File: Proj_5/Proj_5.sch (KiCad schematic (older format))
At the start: 0 parts

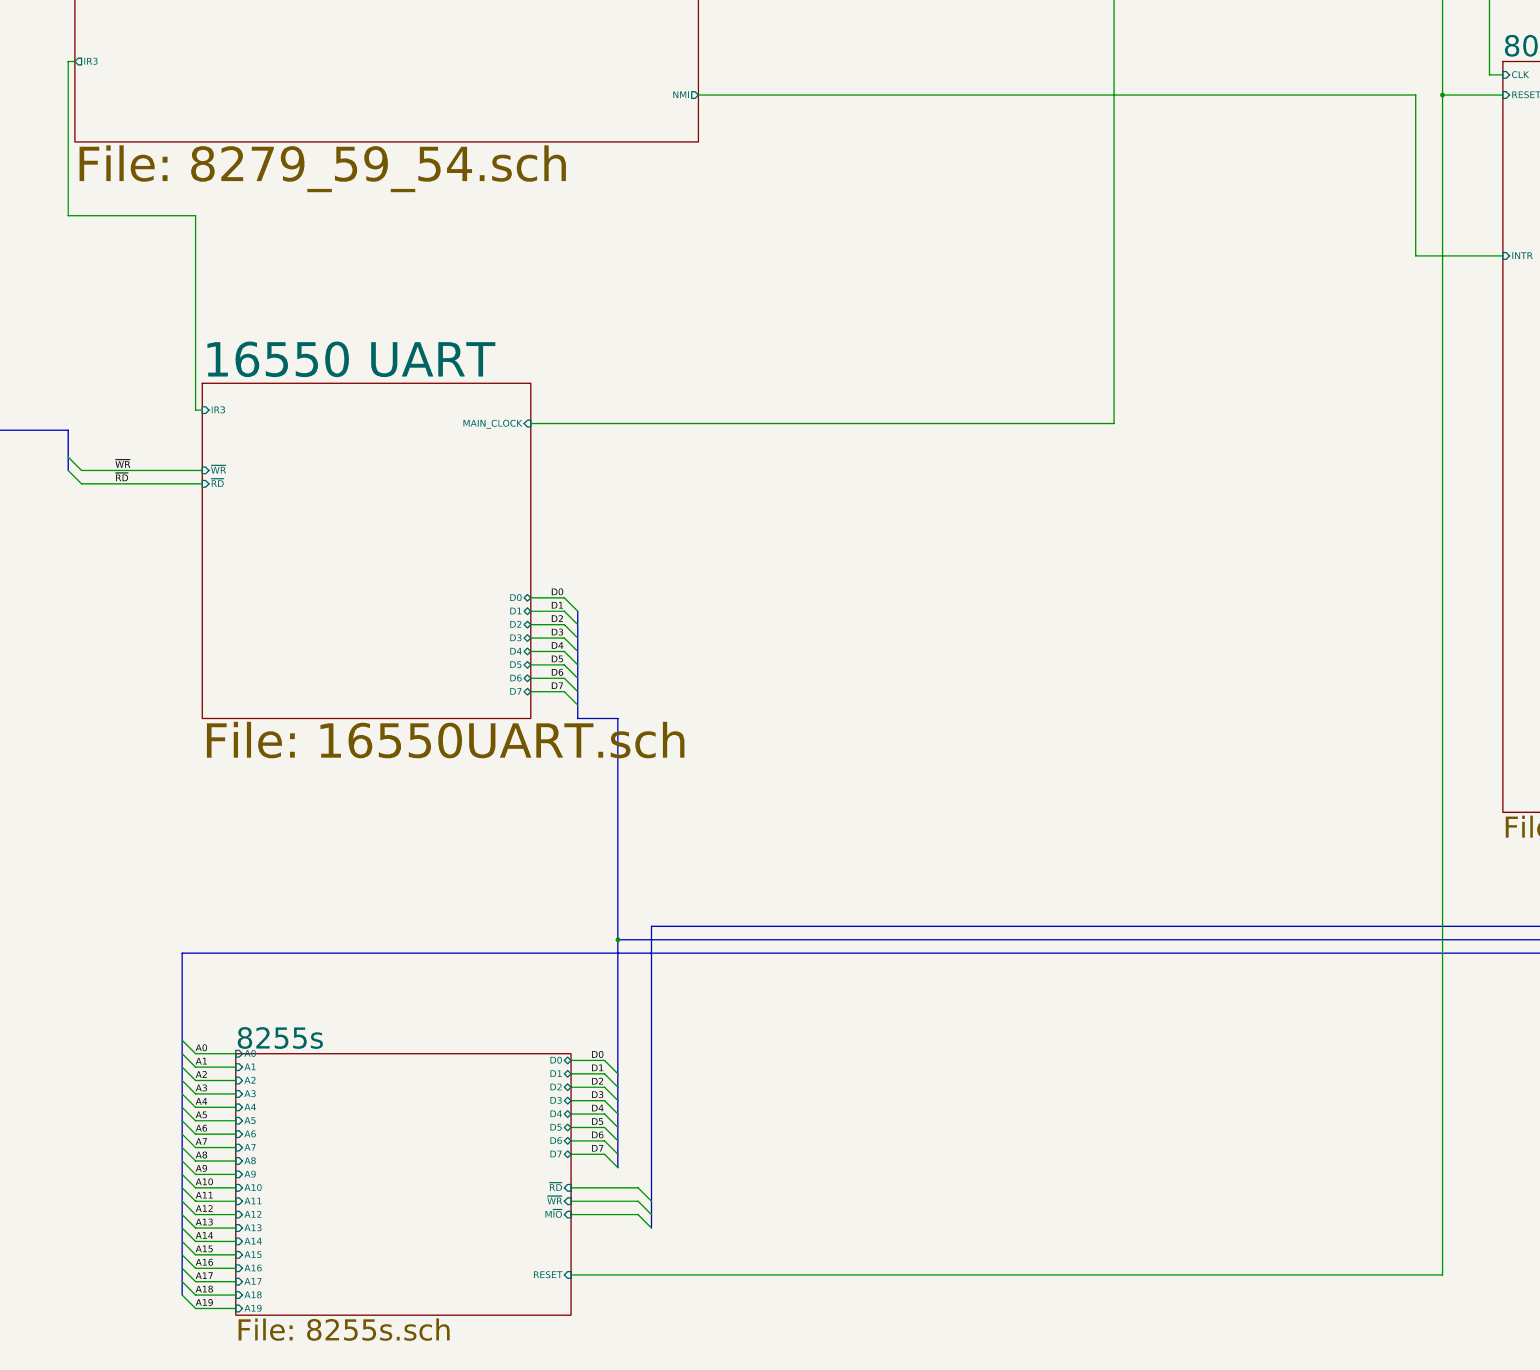
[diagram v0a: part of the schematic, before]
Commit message: Monch
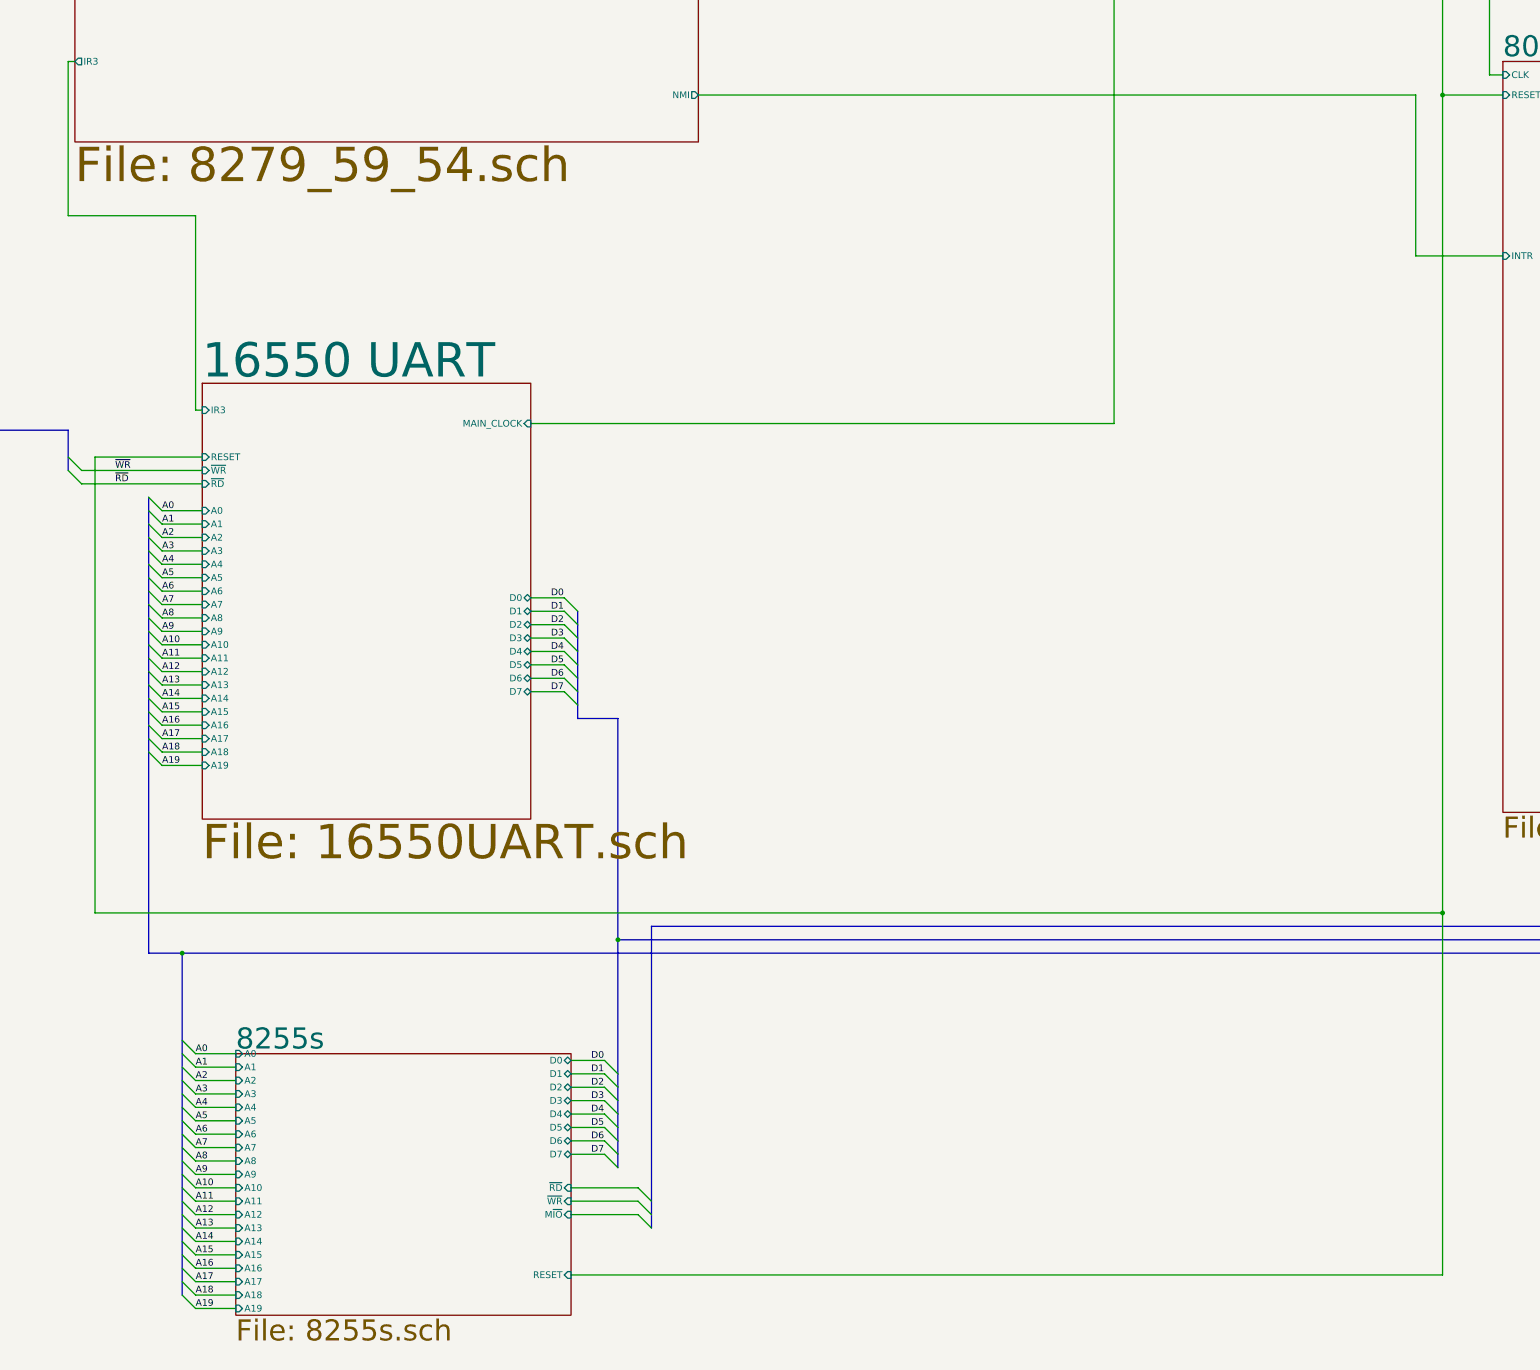
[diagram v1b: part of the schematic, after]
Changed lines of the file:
@@
 	13650 5150 14100 5150
 Wire Wire Line
-	13650 5150 13650 13950
+	13650 5150 13650 11250
 Connection ~ 13650 5150
 Wire Wire Line
 	3450 4900 3400 4900
-$Sheet
-S 4400 7300 2450 2500
-U 5EA98A67
-F0 "16550 UART" 256
-F1 "16550UART.sch" 256
-F2 "MAIN_CLOCK" I R 6850 7600 50
-F3 "IR3" I L 4400 7500 50
-F4 "~WR" I L 4400 7950 50
-F5 "~RD" I L 4400 8050 50
-F6 "D7" B R 6850 9600 50
-F7 "D6" B R 6850 9500 50
-F8 "D5" B R 6850 9400 50
-F9 "D4" B R 6850 9300 50
-F10 "D3" B R 6850 9200 50
-F11 "D2" B R 6850 9100 50
-F12 "D1" B R 6850 9000 50
-F13 "D0" B R 6850 8900 50
-$EndSheet
 Wire Wire Line
 	7150 13950 13650 13950
@@
 	7500 9800 7200 9800
 Connection ~ 7500 11450
+$Sheet
+S 4400 7300 2450 3250
+U 5EA98A67
+F0 "16550 UART" 256
+F1 "16550UART.sch" 256
+F2 "MAIN_CLOCK" I R 6850 7600 50
+F3 "IR3" I L 4400 7500 50
+F4 "~WR" I L 4400 7950 50
+F5 "~RD" I L 4400 8050 50
+F6 "D7" B R 6850 9600 50
+F7 "D6" B R 6850 9500 50
+F8 "D5" B R 6850 9400 50
+F9 "D4" B R 6850 9300 50
+F10 "D3" B R 6850 9200 50
+F11 "D2" B R 6850 9100 50
+F12 "D1" B R 6850 9000 50
+F13 "D0" B R 6850 8900 50
+F14 "RESET" I L 4400 7850 50
+F15 "A1" I L 4400 8350 50
+F16 "A2" I L 4400 8450 50
+F17 "A3" I L 4400 8550 50
+F18 "A4" I L 4400 8650 50
+F19 "A5" I L 4400 8750 50
+F20 "A6" I L 4400 8850 50
+F21 "A7" I L 4400 8950 50
+F22 "A8" I L 4400 9050 50
+F23 "A9" I L 4400 9150 50
+F24 "A10" I L 4400 9250 50
+F25 "A11" I L 4400 9350 50
+F26 "A12" I L 4400 9450 50
+F27 "A13" I L 4400 9550 50
+F28 "A14" I L 4400 9650 50
+F29 "A15" I L 4400 9750 50
+F30 "A0" I L 4400 8250 50
+F31 "A16" I L 4400 9850 50
+F32 "A17" I L 4400 9950 50
+F33 "A18" I L 4400 10050 50
+F34 "A19" I L 4400 10150 50
+$EndSheet
+Entry Wire Line
+	4000 10050 4100 10150
+Entry Wire Line
+	4000 9950 4100 10050
+Entry Wire Line
+	4000 9850 4100 9950
+Entry Wire Line
+	4000 9750 4100 9850
+Entry Wire Line
+	4000 9650 4100 9750
+Entry Wire Line
+	4000 9550 4100 9650
+Entry Wire Line
+	4000 9450 4100 9550
+Entry Wire Line
+	4000 9350 4100 9450
+Entry Wire Line
+	4000 9250 4100 9350
+Entry Wire Line
+	4000 9150 4100 9250
+Entry Wire Line
+	4000 9050 4100 9150
+Entry Wire Line
+	4000 8950 4100 9050
+Entry Wire Line
+	4000 8850 4100 8950
+Entry Wire Line
+	4000 8750 4100 8850
+Entry Wire Line
+	4000 8650 4100 8750
+Entry Wire Line
+	4000 8550 4100 8650
+Entry Wire Line
+	4000 8450 4100 8550
+Entry Wire Line
+	4000 8150 4100 8250
+Wire Wire Line
+	4100 8550 4400 8550
+Wire Wire Line
+	4100 8650 4400 8650
+Wire Wire Line
+	4100 8750 4400 8750
+Wire Wire Line
+	4100 8850 4400 8850
+Wire Wire Line
+	4100 8950 4400 8950
+Wire Wire Line
+	4100 9050 4400 9050
+Wire Wire Line
+	4100 9150 4400 9150
+Wire Wire Line
+	4100 9250 4400 9250
+Wire Wire Line
+	4100 9350 4400 9350
+Wire Wire Line
+	4100 9450 4400 9450
+Wire Wire Line
+	4100 9550 4400 9550
+Wire Wire Line
+	4100 9650 4400 9650
+Wire Wire Line
+	4100 9750 4400 9750
+Wire Wire Line
+	4100 9850 4400 9850
+Wire Wire Line
+	4100 9950 4400 9950
+Wire Wire Line
+	4100 10050 4400 10050
+Wire Wire Line
+	4100 10150 4400 10150
+Text Label 4100 8250 0    50   ~ 0
+A0
+Text Label 4100 8650 0    50   ~ 0
+A4
+Text Label 4100 8750 0    50   ~ 0
+A5
+Text Label 4100 8850 0    50   ~ 0
+A6
+Text Label 4100 8950 0    50   ~ 0
+A7
+Text Label 4100 9050 0    50   ~ 0
+A8
+Text Label 4100 9150 0    50   ~ 0
+A9
+Text Label 4100 9250 0    50   ~ 0
+A10
+Text Label 4100 9350 0    50   ~ 0
+A11
+Text Label 4100 9450 0    50   ~ 0
+A12
+Text Label 4100 9550 0    50   ~ 0
+A13
+Text Label 4100 9650 0    50   ~ 0
+A14
+Text Label 4100 9750 0    50   ~ 0
+A15
+Text Label 4100 9850 0    50   ~ 0
+A16
+Text Label 4100 9950 0    50   ~ 0
+A17
+Text Label 4100 10050 0    50   ~ 0
+A18
+Text Label 4100 10150 0    50   ~ 0
+A19
+Text Label 4100 8550 0    50   ~ 0
+A3
+Wire Wire Line
+	4100 8250 4400 8250
+Entry Wire Line
+	4000 8250 4100 8350
+Entry Wire Line
+	4000 8350 4100 8450
+Wire Wire Line
+	4100 8350 4400 8350
+Wire Wire Line
+	4100 8450 4400 8450
+Text Label 4100 8350 0    50   ~ 0
+A1
+Text Label 4100 8450 0    50   ~ 0
+A2
+Wire Bus Line
+	4250 11550 4000 11550
+Connection ~ 4250 11550
+Wire Wire Line
+	13650 11250 3600 11250
+Wire Wire Line
+	3600 11250 3600 7850
+Wire Wire Line
+	3600 7850 4400 7850
 Wire Bus Line
 	3400 7650 3400 7950
@@
 	16950 9800 16950 10250
 Wire Bus Line
+	7200 9000 7200 9800
+Wire Bus Line
 	8700 1750 8700 3100
 Wire Bus Line
@@
 	28450 2250 28450 8250
 Wire Bus Line
-	7200 9000 7200 9800
-Wire Bus Line
 	17000 4900 17000 6400
 Wire Bus Line
@@
 Wire Bus Line
 	4250 11550 4250 14100
+Wire Bus Line
+	4000 8150 4000 11550
+Connection ~ 13650 11250
+Wire Wire Line
+	13650 11250 13650 13950
 $EndSCHEMATC
